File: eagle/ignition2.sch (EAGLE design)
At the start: 21 parts, among them IC1 LM358N, IC2 NE555, J1 PIN2F061.100, J2 PIN2F061.100, J3 PIN2F061.100, J4 PIN2F061.100, Q1 MJ2955, T1 2N3055

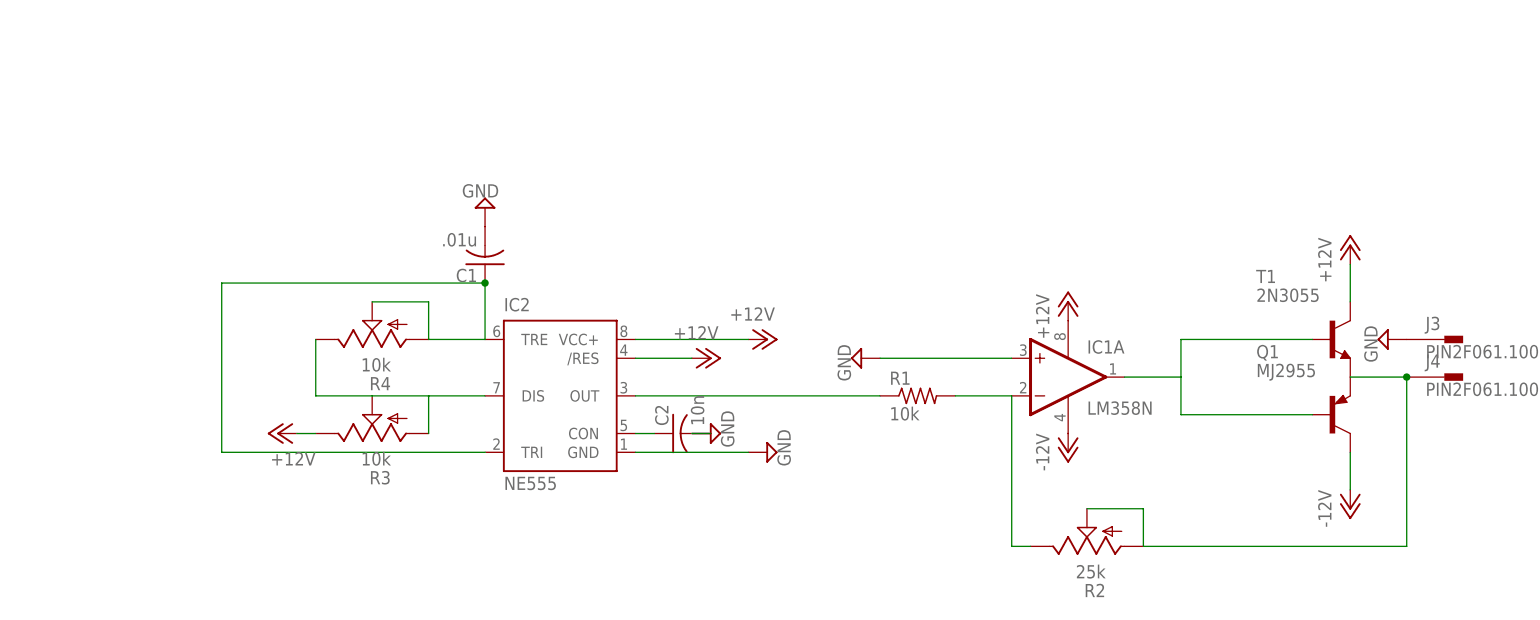
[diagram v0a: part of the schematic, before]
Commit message: BOARDS
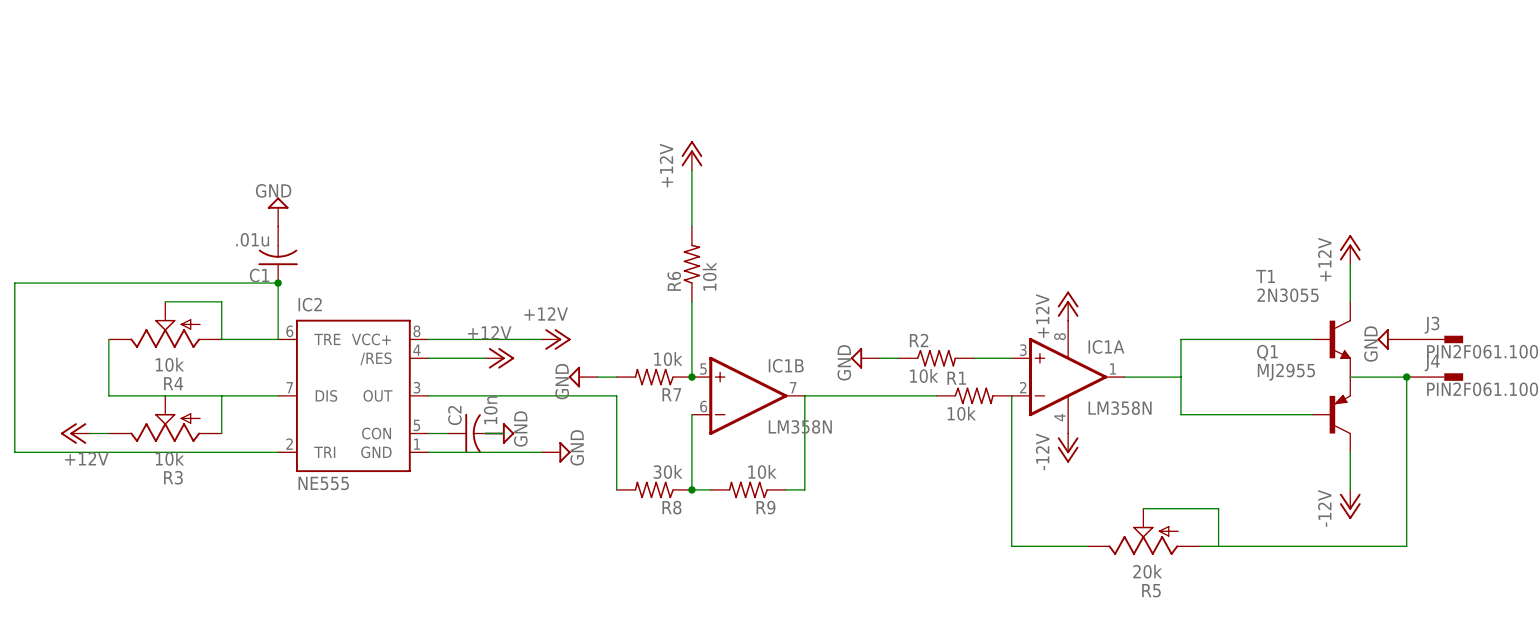
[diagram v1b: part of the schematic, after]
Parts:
- added R5: 20k, pot:TRIM_US-RJ9W
- added R6: 10k, resistor:R-US_0207/12
- added R7, R9: 10k, resistor:R-US_0207/10
- added R8: 30k, resistor:R-US_0207/10
- C1: device rcl:C-US050-035X075 -> rcl:C-US075-042X103
- R1: device resistor:R-US_0207/10 -> resistor:R-US_0207/15
- R2: value 25k -> 10k; device pot:TRIM_US-B64Y -> resistor:R-US_0207/15
- R3, R4: device pot:TRIM_US-B64Y -> pot:TRIM_US-RJ9W
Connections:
- new net N$10: IC1B.+IN, R6.1, R7.1
- new net N$11: IC1B.-IN, R8.1, R9.2
- new net N$12: IC2.OUT, R8.2
- new net N$9: IC1A.+IN, R2.2
- net +12V: now also R6.2
- net GND: now also R2.1, R7.2; no longer IC1A.+IN
- net N$1: now also R5.E; no longer R2.E
- net N$3: now also R5.A, R5.S; no longer R2.A, R2.S
- net N$4: now also IC1B.OUT, R9.1; no longer IC2.OUT
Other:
- moved on the sheet: C1, C2, IC2, R1, R3, R4
